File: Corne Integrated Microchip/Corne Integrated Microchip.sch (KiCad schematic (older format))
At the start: 44 parts, among them J1 MJ-4PP-9, J2 MJ-4PP-9, SW1 SW_Push, SW2 SW_Push, U1 ATmega32U4-AU, U2 ATmega32U4-AU, U3 PRTR5V0U2X, U4 PRTR5V0U2X, Y1 16MHz, Y2 16MHz

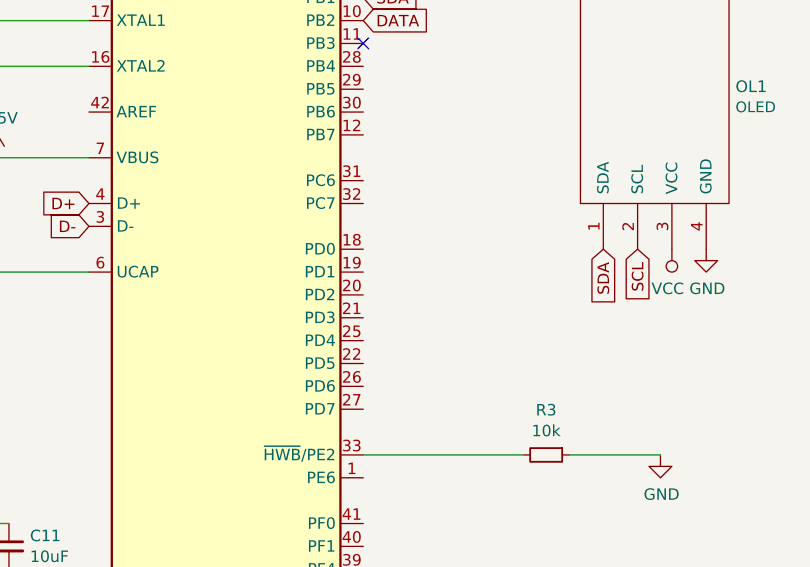
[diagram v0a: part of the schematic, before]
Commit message: continued routing
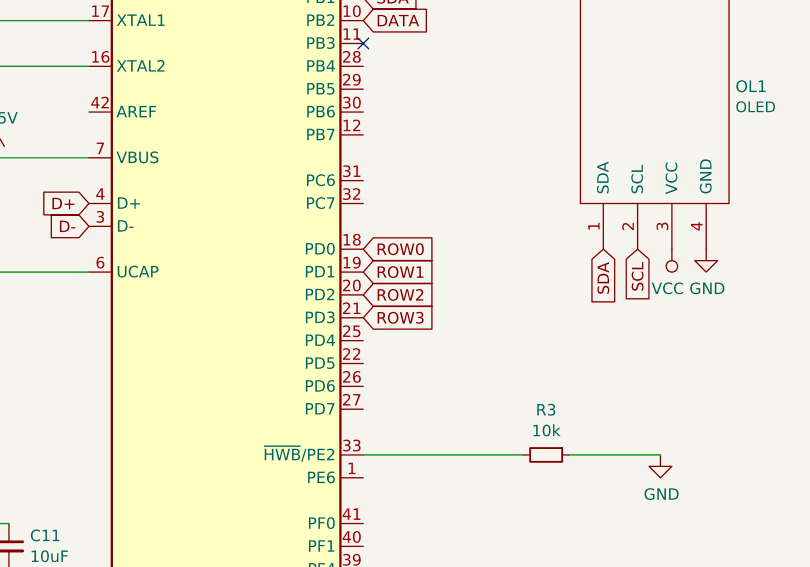
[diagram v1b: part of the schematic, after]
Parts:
- OL1, OL2: footprint kbd:OLED_1side -> kbd:OLED
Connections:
- net ROW0: now reaches U1.18 (PD0)
- net ROW1: now reaches U1.19 (PD1)
- net ROW2: now reaches U1.20 (PD2)
- net ROW3: now reaches U1.21 (PD3)
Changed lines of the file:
@@
 F 0 "OL1" V 5161 1822 51  0000 R CNN
 F 1 "OLED" V 5071 1822 47  0000 R CNN
-F 2 "kbd:OLED_1side" H 5200 2250 60  0001 C CNN
+F 2 "kbd:OLED" H 5200 2250 60  0001 C CNN
 F 3 "" H 5200 2250 60  0001 C CNN
 	1    5200 2150
@@
 F 0 "OL2" V 10411 1822 51  0000 R CNN
 F 1 "OLED" V 10321 1822 47  0000 R CNN
-F 2 "kbd:OLED_1side" H 10450 2250 60  0001 C CNN
+F 2 "kbd:OLED" H 10450 2250 60  0001 C CNN
 F 3 "" H 10450 2250 60  0001 C CNN
 	1    10450 2150
@@
 	1    0    0    -1
 $EndComp
+Text GLabel 3900 2900 2    50   Input ~ 0
+ROW0
+Text GLabel 3900 3000 2    50   Input ~ 0
+ROW1
+Text GLabel 3900 3100 2    50   Input ~ 0
+ROW2
+Text GLabel 3900 3200 2    50   Input ~ 0
+ROW3
 $EndSCHEMATC

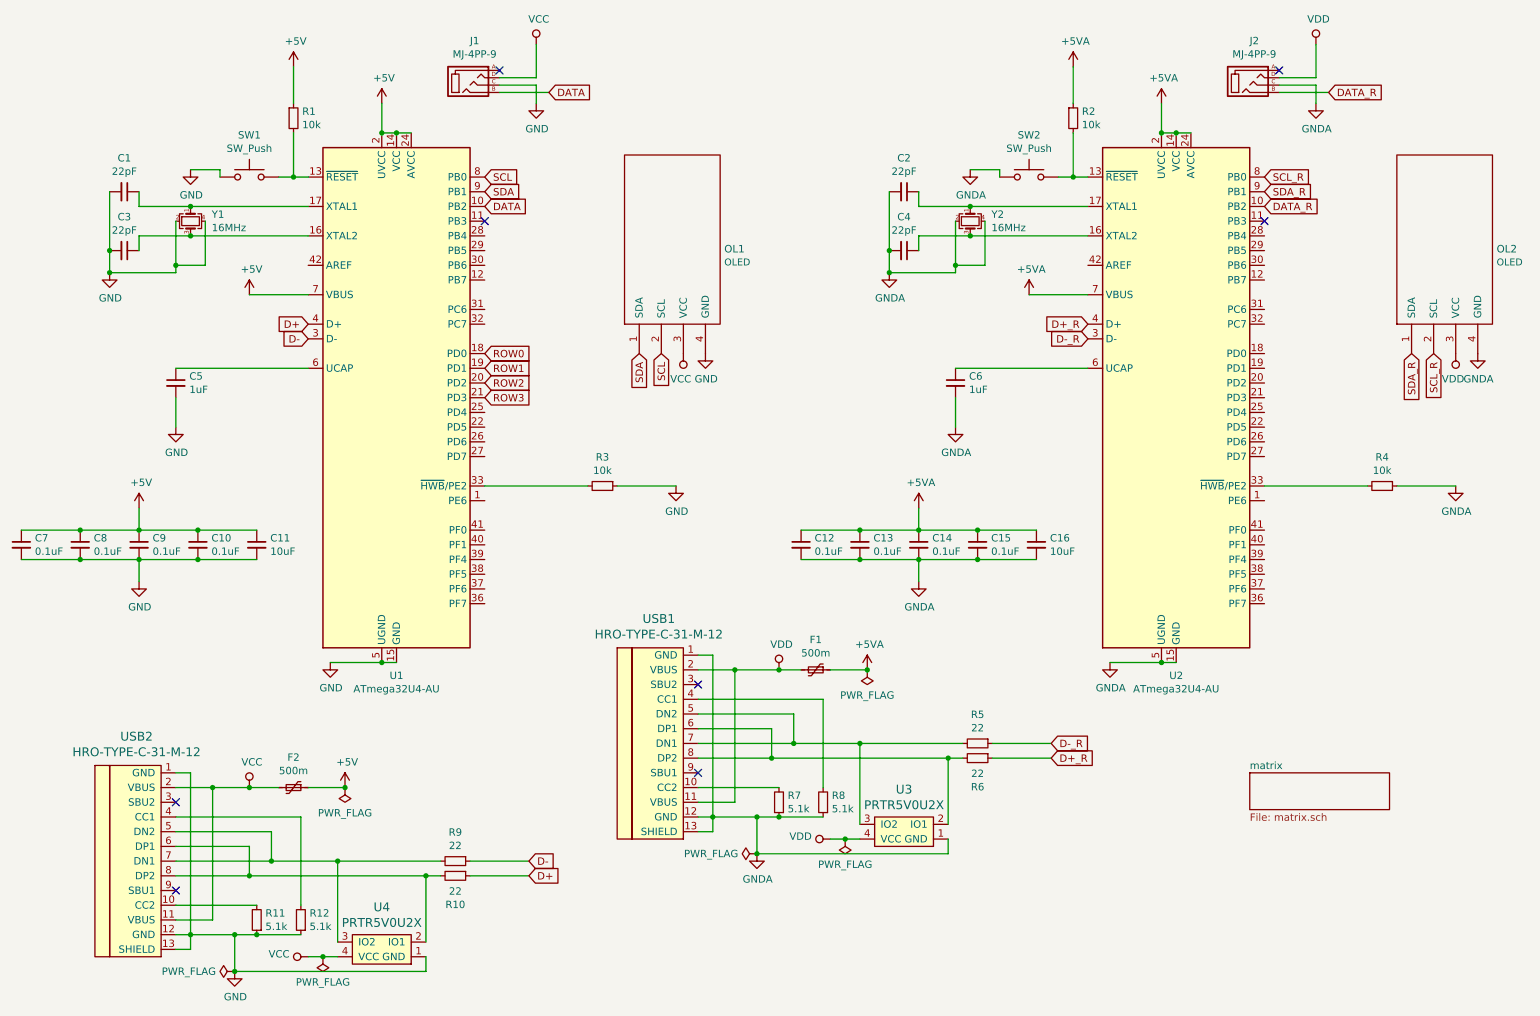
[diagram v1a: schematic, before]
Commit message: Finished routing
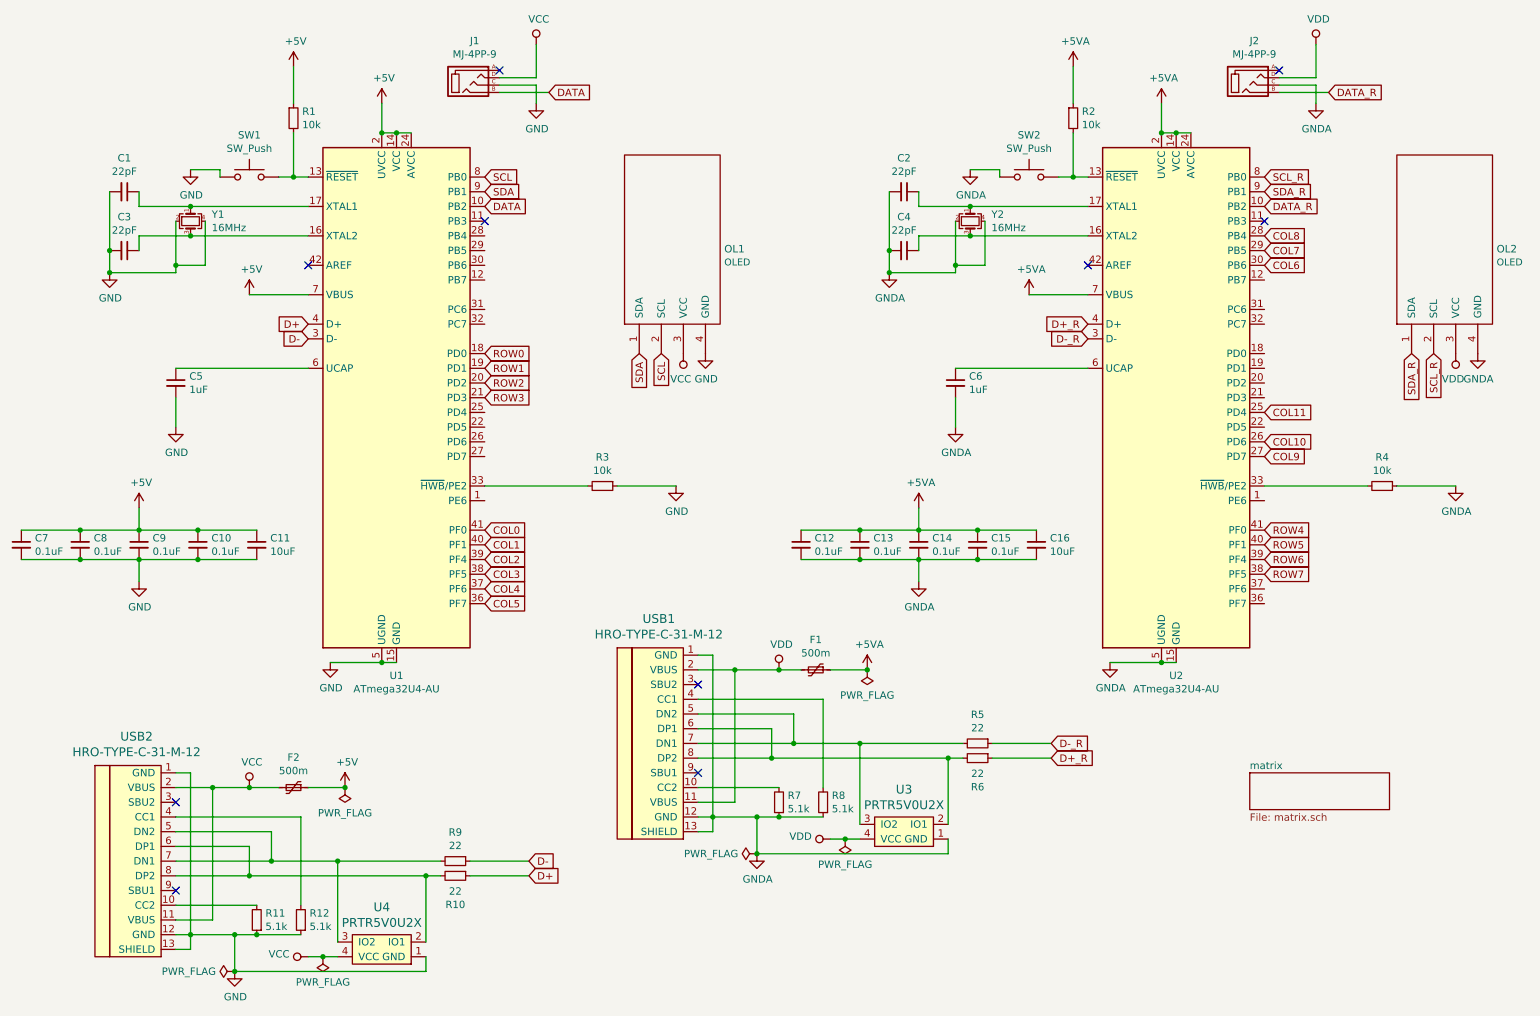
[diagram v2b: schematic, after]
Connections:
- net COL5: now reaches U1.36 (PF7)
- net COL4: now reaches U1.37 (PF6)
- net COL3: now reaches U1.38 (PF5)
- net COL2: now reaches U1.39 (PF4)
- net COL1: now reaches U1.40 (PF1)
- net COL0: now reaches U1.41 (PF0)
- net COL11: now reaches U2.25 (PD4)
- net COL10: now reaches U2.26 (PD6)
- net COL9: now reaches U2.27 (PD7)
- net COL8: now reaches U2.28 (PB4)
- net COL7: now reaches U2.29 (PB5)
- net COL6: now reaches U2.30 (PB6)
- net ROW7: now reaches U2.38 (PF5)
- net ROW6: now reaches U2.39 (PF4)
- net ROW5: now reaches U2.40 (PF1)
- net ROW4: now reaches U2.41 (PF0)
- no-connect marks 8 -> 10
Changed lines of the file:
@@
 Text GLabel 3900 3200 2    50   Input ~ 0
 ROW3
+Text GLabel 3900 4600 2    50   Input ~ 0
+COL5
+Text GLabel 3900 4500 2    50   Input ~ 0
+COL4
+Text GLabel 3900 4400 2    50   Input ~ 0
+COL3
+Text GLabel 3900 4300 2    50   Input ~ 0
+COL2
+Text GLabel 3900 4200 2    50   Input ~ 0
+COL1
+Text GLabel 3900 4100 2    50   Input ~ 0
+COL0
+NoConn ~ 2700 2300
+Text GLabel 9200 2300 2    50   Input ~ 0
+COL6
+Text GLabel 9200 2200 2    50   Input ~ 0
+COL7
+Text GLabel 9200 2100 2    50   Input ~ 0
+COL8
+Text GLabel 9200 3600 2    50   Input ~ 0
+COL9
+Text GLabel 9200 3500 2    50   Input ~ 0
+COL10
+Text GLabel 9200 3300 2    50   Input ~ 0
+COL11
+NoConn ~ 8000 2300
+Text GLabel 9200 4100 2    50   Input ~ 0
+ROW4
+Text GLabel 9200 4200 2    50   Input ~ 0
+ROW5
+Text GLabel 9200 4300 2    50   Input ~ 0
+ROW6
+Text GLabel 9200 4400 2    50   Input ~ 0
+ROW7
 $EndSCHEMATC
